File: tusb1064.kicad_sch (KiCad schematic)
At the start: 28 parts, among them U13 TUSB1064RNQT

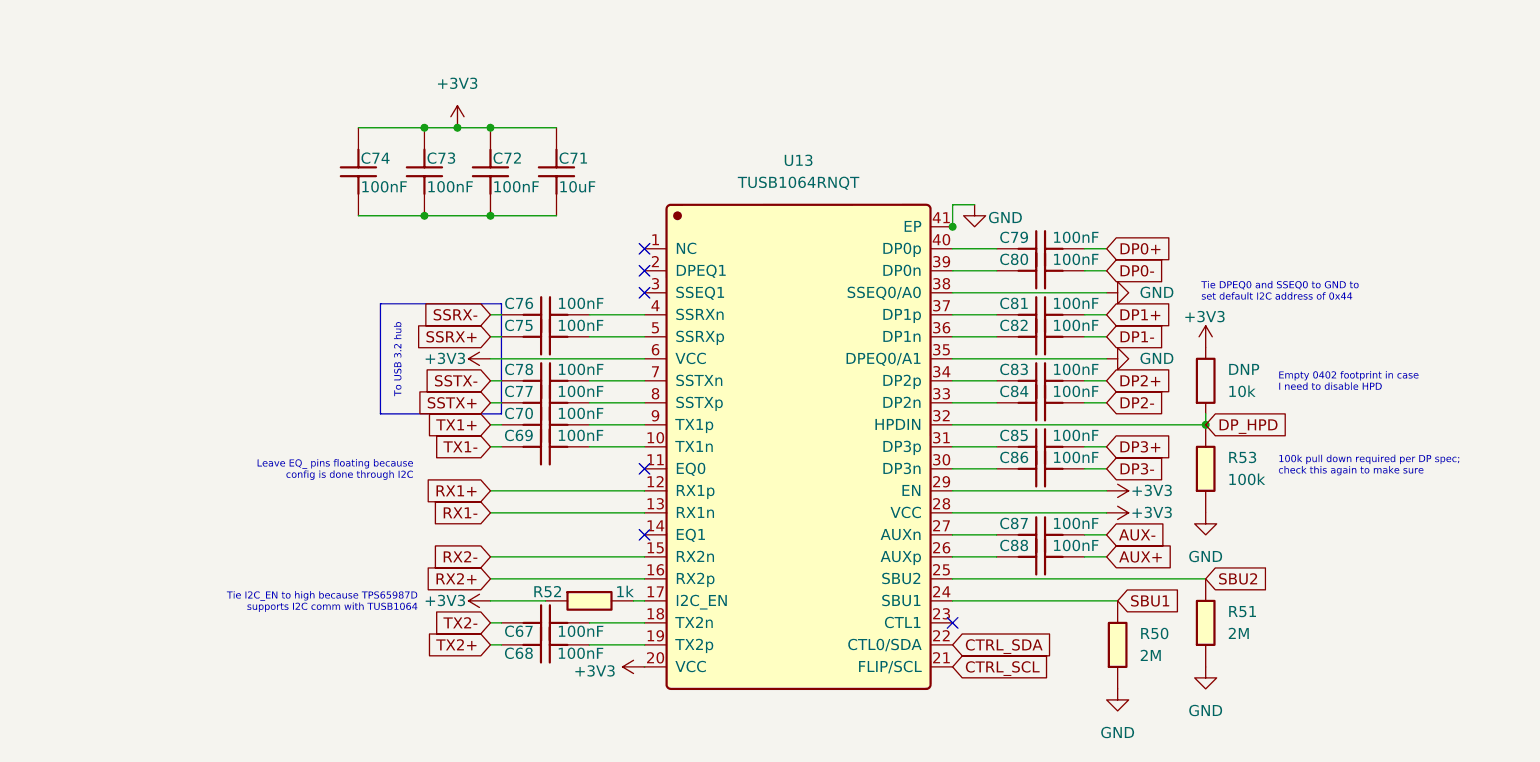
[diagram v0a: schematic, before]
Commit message: Preliminary Revision of PS176 DP->HDMI Subsystem
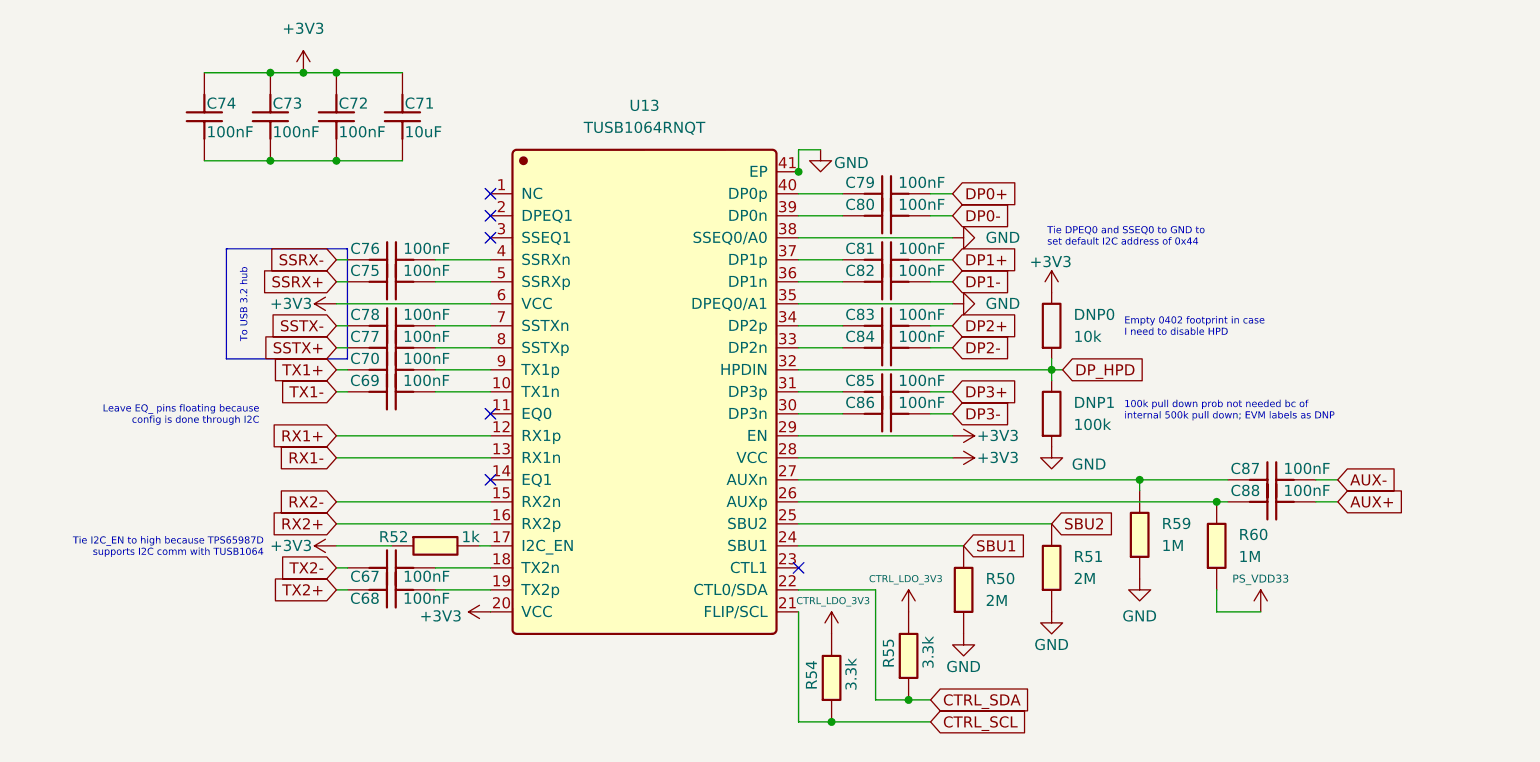
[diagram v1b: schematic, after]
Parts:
- removed R53: 100k, Resistor_SMD:R_0402_1005Metric, symbol JLCImport:0402WGF1003TCE
- added DNP1: 100k, Resistor_SMD:R_01005_0402Metric, symbol Device:R
- added R54, R55: 3.3k, Resistor_SMD:R_0402_1005Metric, symbol JLCImport:0402WGF3301TCE
- added R59, R60: 1M, Resistor_SMD:R_0402_1005Metric, symbol JLCImport:0402WGF1004TCE
- renumbered DNP to DNP0
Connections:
- net CTRL_SCL: now also U13.21 (FLIP/SCL), R54.1
- net CTRL_SDA: now also R55.1
- net DP_HPD: now also DNP1.1
- net GND: now also DNP1.2, R59.1
- net at C87.1, U13.27 (AUXn): now also R59.2
- net at C88.1, U13.26 (AUXp): now also R60.2
- new net CTRL_LDO_3V3: R54.2, R55.2
- new net PS_VDD33: R60.1
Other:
- note added: "100k pull down prob not needed bc of internal 500k pull down; EVM labels as DNP"
- note removed: "100k pull down required per DP spec; check this again to make sure"
- moved on the sheet: C67, C68, C69, C70, C71, C72, C73, C74, C75, C76, C77, C78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
